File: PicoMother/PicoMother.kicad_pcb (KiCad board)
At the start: 2 copper layers, 73.6 x 51.9 mm, 57 parts, among them J1 M20-9980345, J2 Micro_SD, J3 M20-9980345, J4 Conn_02x04_Counter_Clockwise, J5 Conn_02x04_Counter_Clockwise, J6 Conn_02x04_Counter_Clockwise, J7 Conn_02x04_Counter_Clockwise, J8 USB_C, J9 Conn_02x04_Counter_Clockwise, SW1 SW_Push, U1 74LVC125, U2 LM1117-3.3, U4 ATmega328P-A, U5 ATmega8U2-A, Y1 Crystal_GND24, Y4 Crystal_GND24

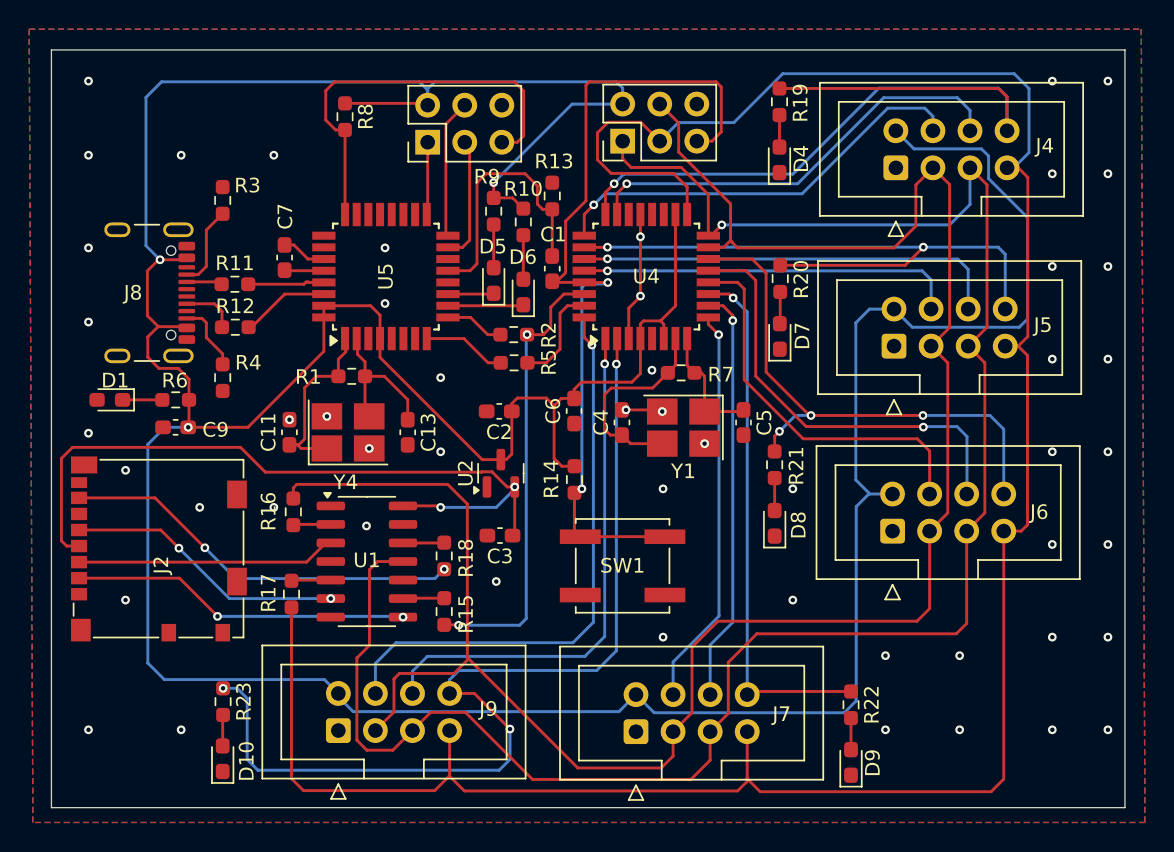
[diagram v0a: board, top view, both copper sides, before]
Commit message: modif schema et routage
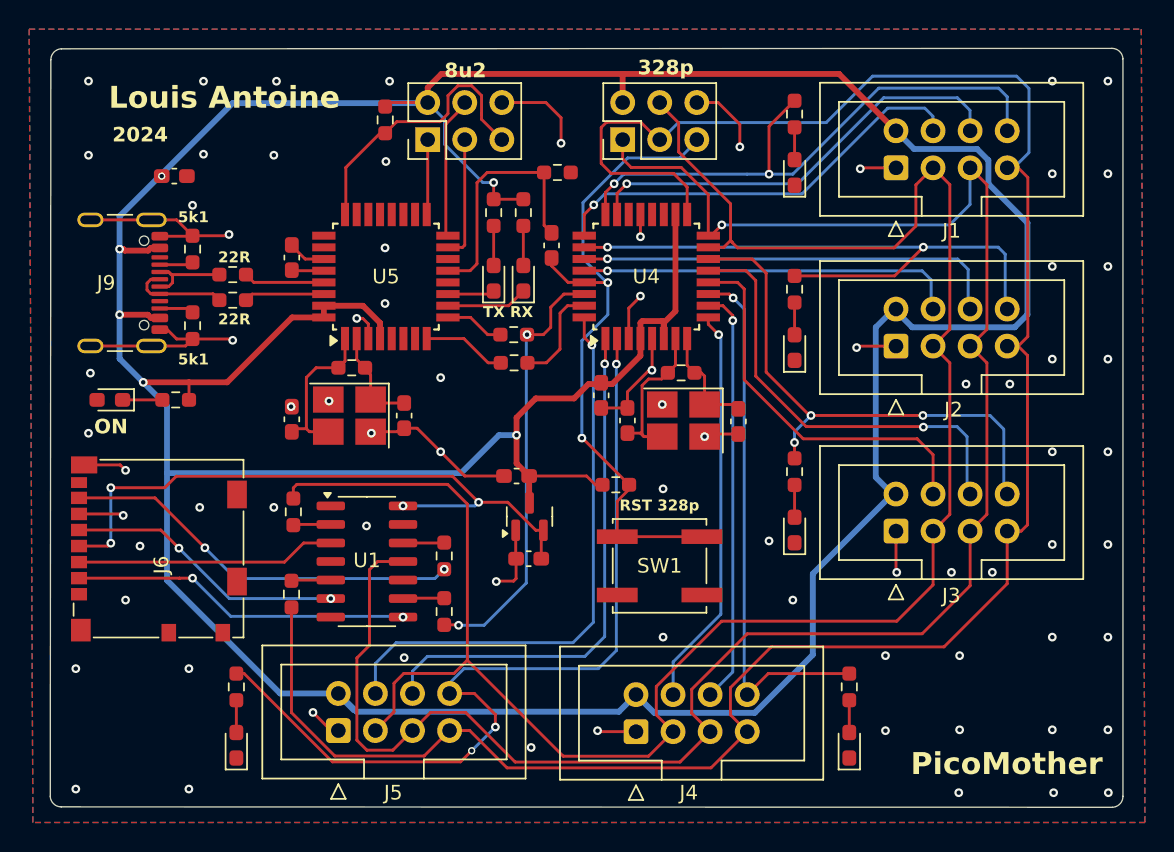
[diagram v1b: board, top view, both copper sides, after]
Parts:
- moved C9 17.2 mm to (108.8, 85.2), turned to 0 degrees
- moved C13 7.99 mm to (116.8, 101.9), turned to 90 degrees
- moved C11 7.94 mm to (124.5, 101.7), turned to -90 degrees
- moved C2 4.58 mm to (132.2, 105.8)
- moved R4 4.12 mm to (110.0, 95.5)
- moved R3 3.92 mm to (110.0, 90.2)
- moved U2 3.56 mm to (133.1, 108.6)
- moved R14 2.85 mm to (139.0, 106.4), turned to 0 degrees
- moved R8 2.76 mm to (123.2, 81.4)
- moved SW1 2.53 mm to (142.0, 112.0)
- moved C3 2.53 mm to (133.0, 111.5)
- moved C6 2.14 mm to (138.0, 100.3)
- moved J9 1.97 mm to (104.1, 92.6)
- moved R12 1.86 mm to (112.8, 93.8)
- moved R13 1.65 mm to (135.0, 85.0), turned to 0 degrees
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- renumbered J4 to J1, J5 to J2, J6 to J3, J7 to J4, J9 to J5, J2 to J6, J3 to J7, J1 to J8, J8 to J9
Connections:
- net CS1_1 renamed CS_SD_3v3
- J1 pad 8: CS2 -> CS1
- J2 pad 8: CS3 -> CS2
- J3 pad 8: CS4 -> CS3
- J4 pad 8: CS5 -> CS4
- J5 pad 8: CS6 -> CS5
- R15 pad 1: CS1 -> CS_SD
- R19 pad 1: CS2 -> CS1
- R2 pad 1: CS1 -> CS_SD
- R20 pad 1: CS3 -> CS2
- R21 pad 1: CS4 -> CS3
- R22 pad 1: CS5 -> CS4
- R23 pad 1: CS6 -> CS5
- U4 pad 11: CS5 -> CS4
- U4 pad 14: CS4 -> CS3
- U4 pad 2: CS6 -> CS5
- U4 pad 24: CS2 -> CS1
- U4 pad 26: CS3 -> CS2
- U4 pad 30: CS1 -> CS_SD
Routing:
- net GND: track 14.3 -> 89.9 mm, vias 52 -> 78
- net CS6: track 66.6 -> 0.00 mm, vias 3 -> 0
- net CS_SD: track 0.00 -> 29.8 mm, vias 0 -> 2
- net CS5: track 36.6 -> 60.3 mm, vias 1 -> 3
- net SCK: track 164.6 -> 149.4 mm
- net USBVCC: track 283.9 -> 298.3 mm, vias 3 -> 6
- net RESET: track 58.3 -> 46.3 mm
- net CS2: track 52.7 -> 42.4 mm, vias 1 -> 2
- net CS1: track 31.2 -> 40.3 mm
- net RESET2: track 28.2 -> 19.5 mm
- net +3V3: track 51.3 -> 44.9 mm, vias 2 -> 4
- net CS3: track 43.1 -> 36.9 mm, vias 2 -> 3
- net Net-(U5-PC0/XTAL2): track 12.3 -> 6.97 mm
- net Net-(J9-D--PadA7): track 2.45 -> 5.99 mm
- net Net-(U4-XTAL1/PB6): track 14.3 -> 10.7 mm
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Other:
- board size 73.6 x 51.9 mm -> 73.5 x 52 mm
- board text added: "2024"
- board text added: "22R"
- board text added: "328p"
- board text added: "5k1"
- board text added: "8u2"
- board text added: "CS1"
- board text added: "CS2"
- board text added: "CS3"
- board text added: "CS4"
- board text added: "CS5"
- board text added: "GND"
- board text added: "INT1"
- board text added: "INT2"
- board text added: "INT3"
- board text added: "INT4"
- board text added: "INT5"
- board text added: "J1"
- board text added: "J2"
- board text added: "J3"
- board text added: "J4"
- board text added: "J5"
- board text added: "Louis Antoine"
- board text added: "MISO"
- board text added: "MOSI"
- board text added: "ON"
- board text added: "PicoMother"
- board text added: "RST"
- board text added: "RST 328p"
- board text added: "RST1"
- board text added: "RST2"
- board text added: "RST3"
- board text added: "RST4"
- board text added: "RST5"
- board text added: "RX"
- board text added: "SCK"
- board text added: "TX"
- board text added: "VCC"
